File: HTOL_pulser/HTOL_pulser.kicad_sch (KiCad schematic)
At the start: 25 parts, among them IC1 4093D, J1 IN_ON, J10 OUT_OFF, J11 OUT_ON, J12 IN_ON, J2 OUT_ON, J3 OUT_OFF, J4 IN_OFF, J5 GND, J6 +5V, J7 +5V, J8 GND, J9 IN_OFF, U1 74AHCT123

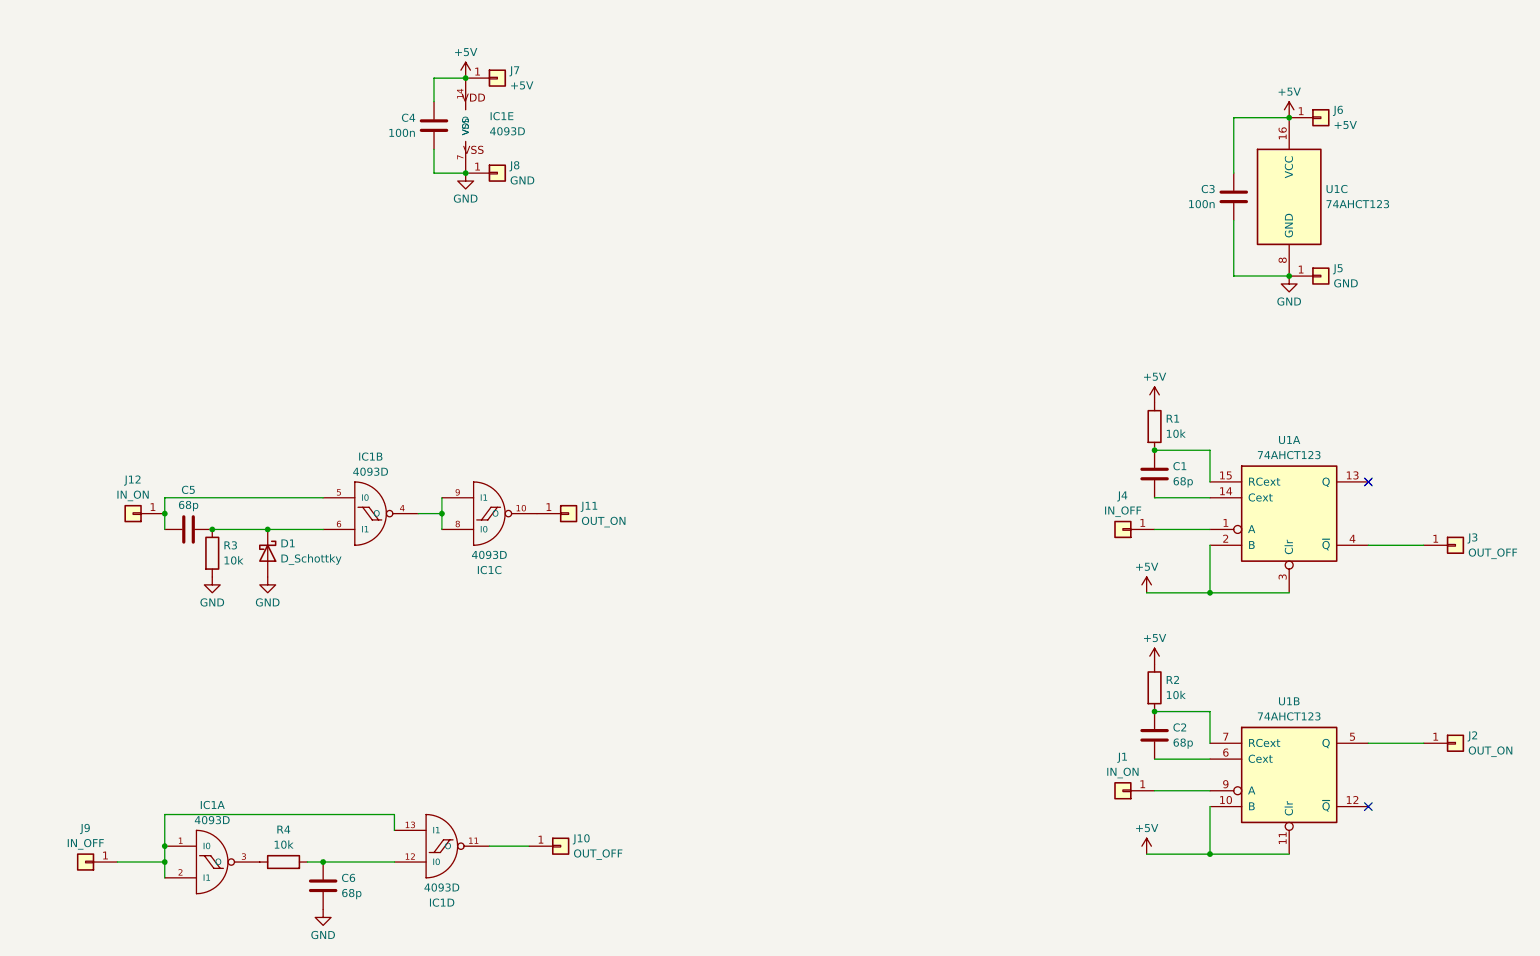
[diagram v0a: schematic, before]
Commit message: a
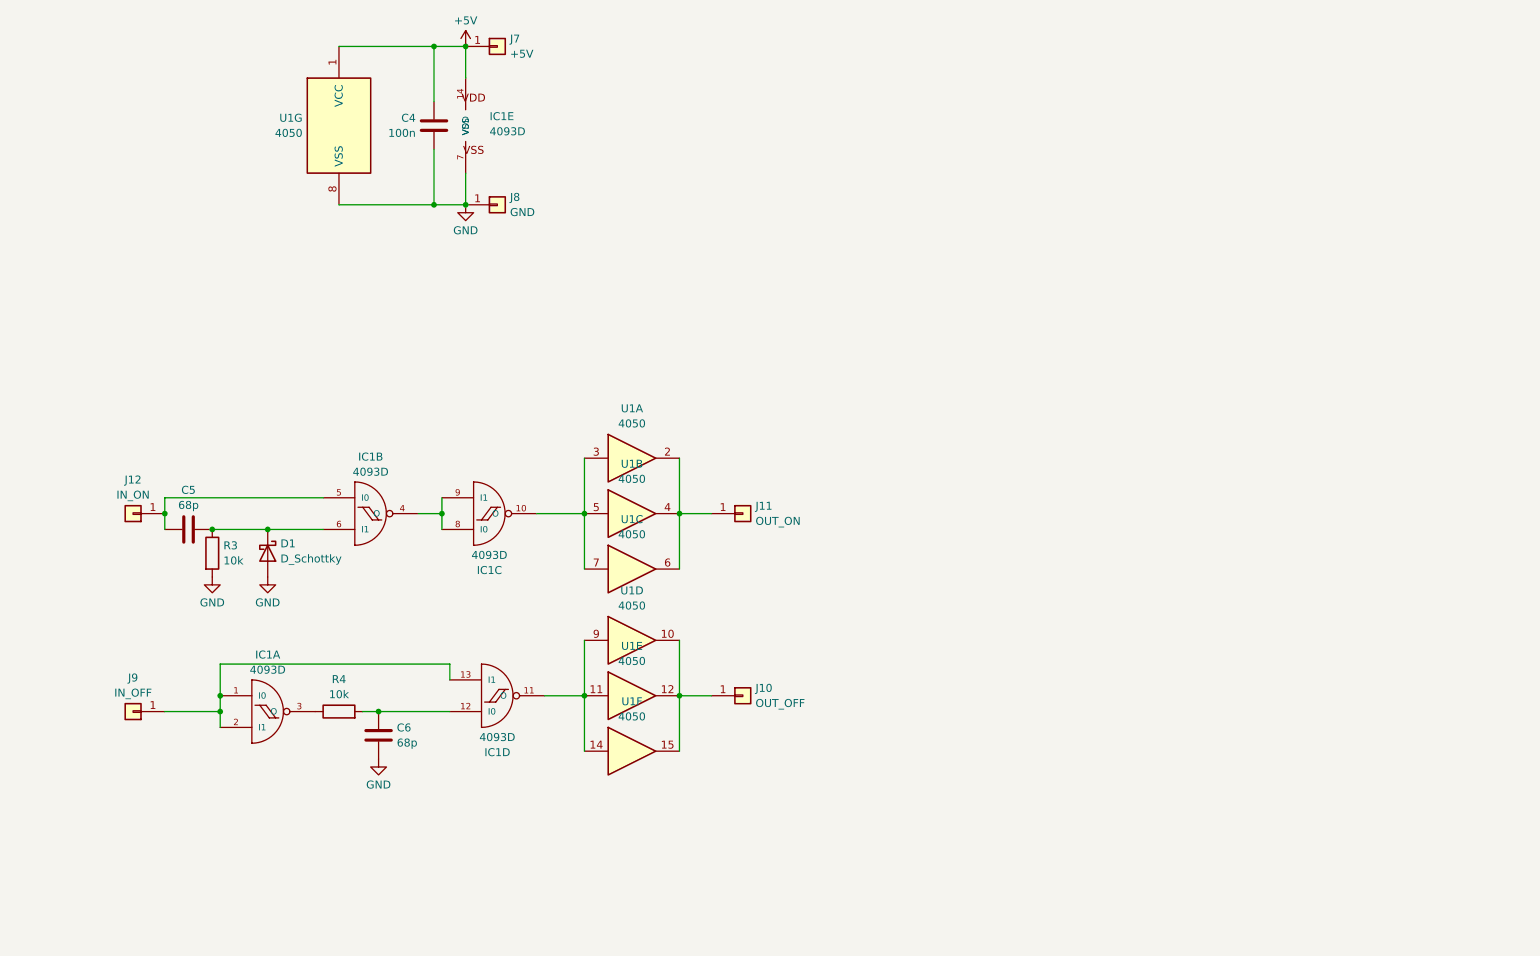
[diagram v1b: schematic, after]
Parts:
- removed C1, C2: 68p, Capacitor_THT:C_Disc_D4.7mm_W2.5mm_P5.00mm, symbol Device:C
- removed C3: 100n, Capacitor_THT:C_Disc_D4.7mm_W2.5mm_P5.00mm, symbol Device:C
- removed J1: IN_ON, Connector_PinHeader_2.54mm:PinHeader_1x01_P2.54mm_Vertical, symbol Connector_Generic:Conn_01x01
- removed J2: OUT_ON, Connector_PinHeader_2.54mm:PinHeader_1x01_P2.54mm_Vertical, symbol Connector_Generic:Conn_01x01
- removed J3: OUT_OFF, Connector_PinHeader_2.54mm:PinHeader_1x01_P2.54mm_Vertical, symbol Connector_Generic:Conn_01x01
- removed J4: IN_OFF, Connector_PinHeader_2.54mm:PinHeader_1x01_P2.54mm_Vertical, symbol Connector_Generic:Conn_01x01
- removed J5: GND, Connector_PinHeader_2.54mm:PinHeader_1x01_P2.54mm_Vertical, symbol Connector_Generic:Conn_01x01
- removed J6: +5V, Connector_PinHeader_2.54mm:PinHeader_1x01_P2.54mm_Vertical, symbol Connector_Generic:Conn_01x01
- removed R1, R2: 10k, Resistor_THT:R_Axial_DIN0207_L6.3mm_D2.5mm_P2.54mm_Vertical, symbol Device:R
- removed U1: 74AHCT123, Package_DIP:DIP-16_W7.62mm_LongPads, symbol 74xx:74AHCT123
- added U1: 4050, Package_DIP:DIP-14_W7.62mm_LongPads, symbol 4xxx:4050
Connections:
- net +5V: now also U1.1 (VCC)
- net GND: now also U1.8 (VSS)
- net at J11.1 (Pin_1): now also U1.2, U1.4, U1.6; no longer IC1.10 (O)
- net at IC1.11 (O): now also U1.11, U1.14, U1.9; no longer J10.1 (Pin_1)
- new net: J10.1 (Pin_1), U1.10, U1.12, U1.15
- new net: IC1.10 (O), U1.3, U1.5, U1.7
- no-connect marks 2 -> 0
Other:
- moved on the sheet: C6, IC1A, IC1D, J10, J11, J7, J8, J9, R4

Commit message: a
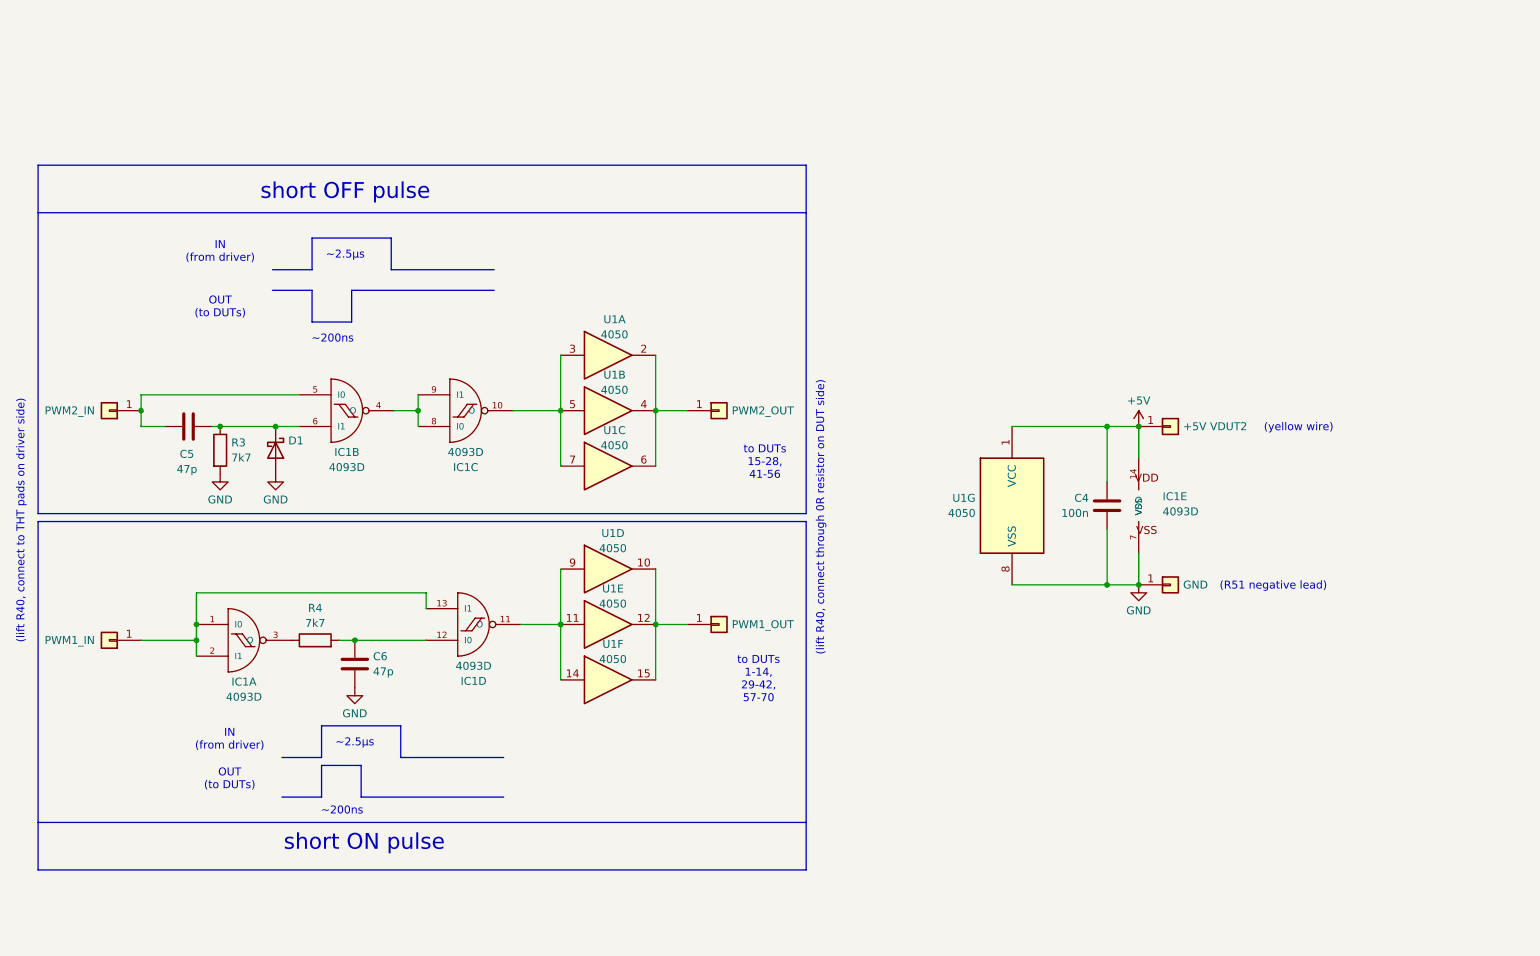
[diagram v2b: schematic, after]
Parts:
- C5, C6: value 68p -> 47p
- J10: value OUT_OFF -> PWM1_OUT
- J11: value OUT_ON -> PWM2_OUT
- J12: value IN_ON -> PWM2_IN
- J7: value +5V -> +5V VDUT2
- J9: value IN_OFF -> PWM1_IN
- R3, R4: value 10k -> 7k7
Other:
- note added: "(R51 negative lead)"
- note added: "(lift R40, connect through 0R resistor on DUT side)"
- note added: "(lift R40, connect to THT pads on driver side)"
- note added: "(yellow wire)"
- note added: "IN (from driver)"
- note added: "OUT (to DUTs)"
- note added: "short OFF pulse"
- note added: "short ON pulse"
- note added: "to DUTs 1-14, 29-42, 57-70"
- note added: "to DUTs 15-28, 41-56"
- note added: "~2.5µs"
- note added: "~200ns"
- title: HTOL pulser -> HTOL short pulse mod
- moved on the sheet: C4, C5, C6, D1, IC1A, IC1B, IC1C, IC1D, IC1E, R3, R4, U1A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
